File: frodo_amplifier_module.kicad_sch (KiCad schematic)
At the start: 19 parts, among them IC1 INA826AID, IC2 AS321KTR-G1, J1 Conn_01x01_Socket, J2 Conn_01x01_Socket, J3 Conn_01x01_Socket, J4 Conn_01x01_Socket, J5 Conn_01x01_Socket, J6 Conn_01x01_Socket, J7 Conn_01x01_Socket, J8 Conn_01x01_Socket

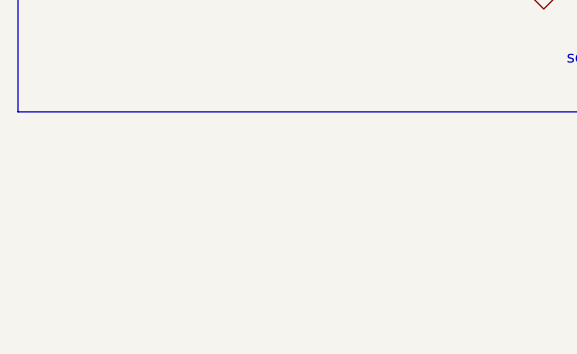
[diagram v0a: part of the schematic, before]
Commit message: added stuff
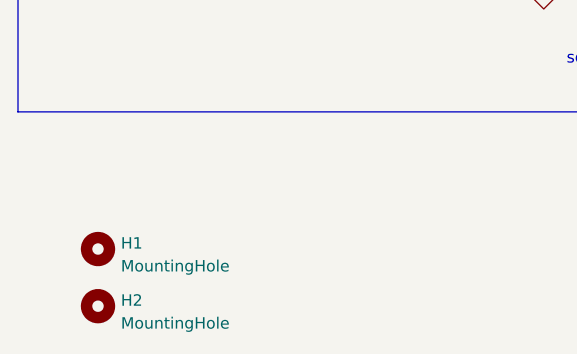
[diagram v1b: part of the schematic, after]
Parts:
- added H1, H2: MountingHole, MountingHole:MountingHole_3.2mm_M3, symbol Mechanical:MountingHole
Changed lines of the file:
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@@
+    )
+  )
+  (symbol (lib_id "Mechanical:MountingHole") (at 39.37 171.45 0) (unit 1)
+    (in_bom yes) (on_board yes) (dnp no) (fields_autoplaced)
+    (property "Reference" "H1" (at 41.91 170.815 0)
+      (effects (font (size 1.27 1.27)) (justify left))
+    )
+    (property "Value" "MountingHole" (at 41.91 173.355 0)
+      (effects (font (size 1.27 1.27)) (justify left))
+    )
+    (property "Footprint" "MountingHole:MountingHole_3.2mm_M3" (at 39.37 171.45 0)
+      (effects (font (size 1.27 1.27)) hide)
+    )
+    (property "Datasheet" "~" (at 39.37 171.45 0)
+      (effects (font (size 1.27 1.27)) hide)
+    )
+    (instances
+      (project "frodo_amplifier_module"
+        (path "/61190ca3-2171-4daf-b151-7360302be40b"
+          (reference "H1") (unit 1)
+        )
+      )
     )
   )
@@
         )
       )
+    )
+  )
+  (symbol (lib_id "Mechanical:MountingHole") (at 39.37 177.8 0) (unit 1)
+    (in_bom yes) (on_board yes) (dnp no) (fields_autoplaced)
+    (property "Reference" "H2" (at 41.91 177.165 0)
+      (effects (font (size 1.27 1.27)) (justify left))
+    )
+    (property "Value" "MountingHole" (at 41.91 179.705 0)
+      (effects (font (size 1.27 1.27)) (justify left))
+    )
+    (property "Footprint" "MountingHole:MountingHole_3.2mm_M3" (at 39.37 177.8 0)
+      (effects (font (size 1.27 1.27)) hide)
+    )
+    (property "Datasheet" "~" (at 39.37 177.8 0)
+      (effects (font (size 1.27 1.27)) hide)
+    )
+    (instances
+      (project "frodo_amplifier_module"
+        (path "/61190ca3-2171-4daf-b151-7360302be40b"
+          (reference "H2") (unit 1)
+        )
+      )
